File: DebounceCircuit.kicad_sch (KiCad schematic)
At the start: 20 parts, among them U2 74HC14

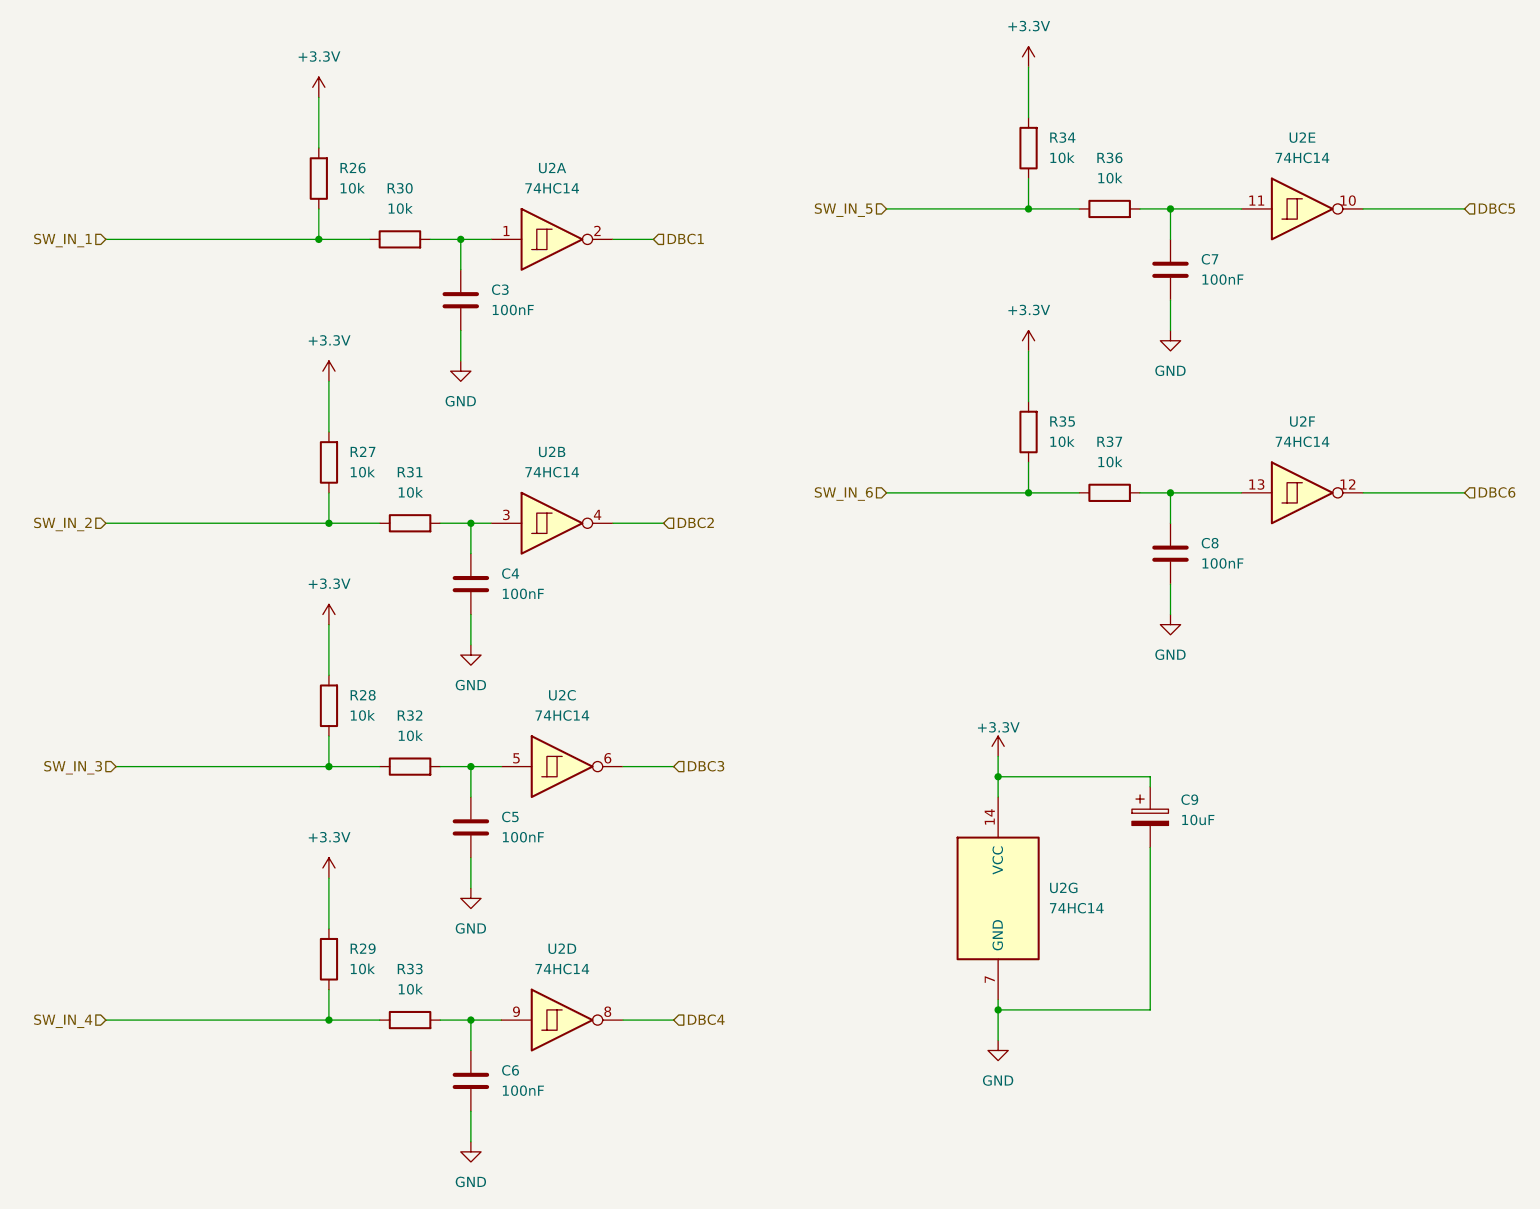
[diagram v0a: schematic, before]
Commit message: Corrigido o botão de seleção de Clock e valores dos capacitores.
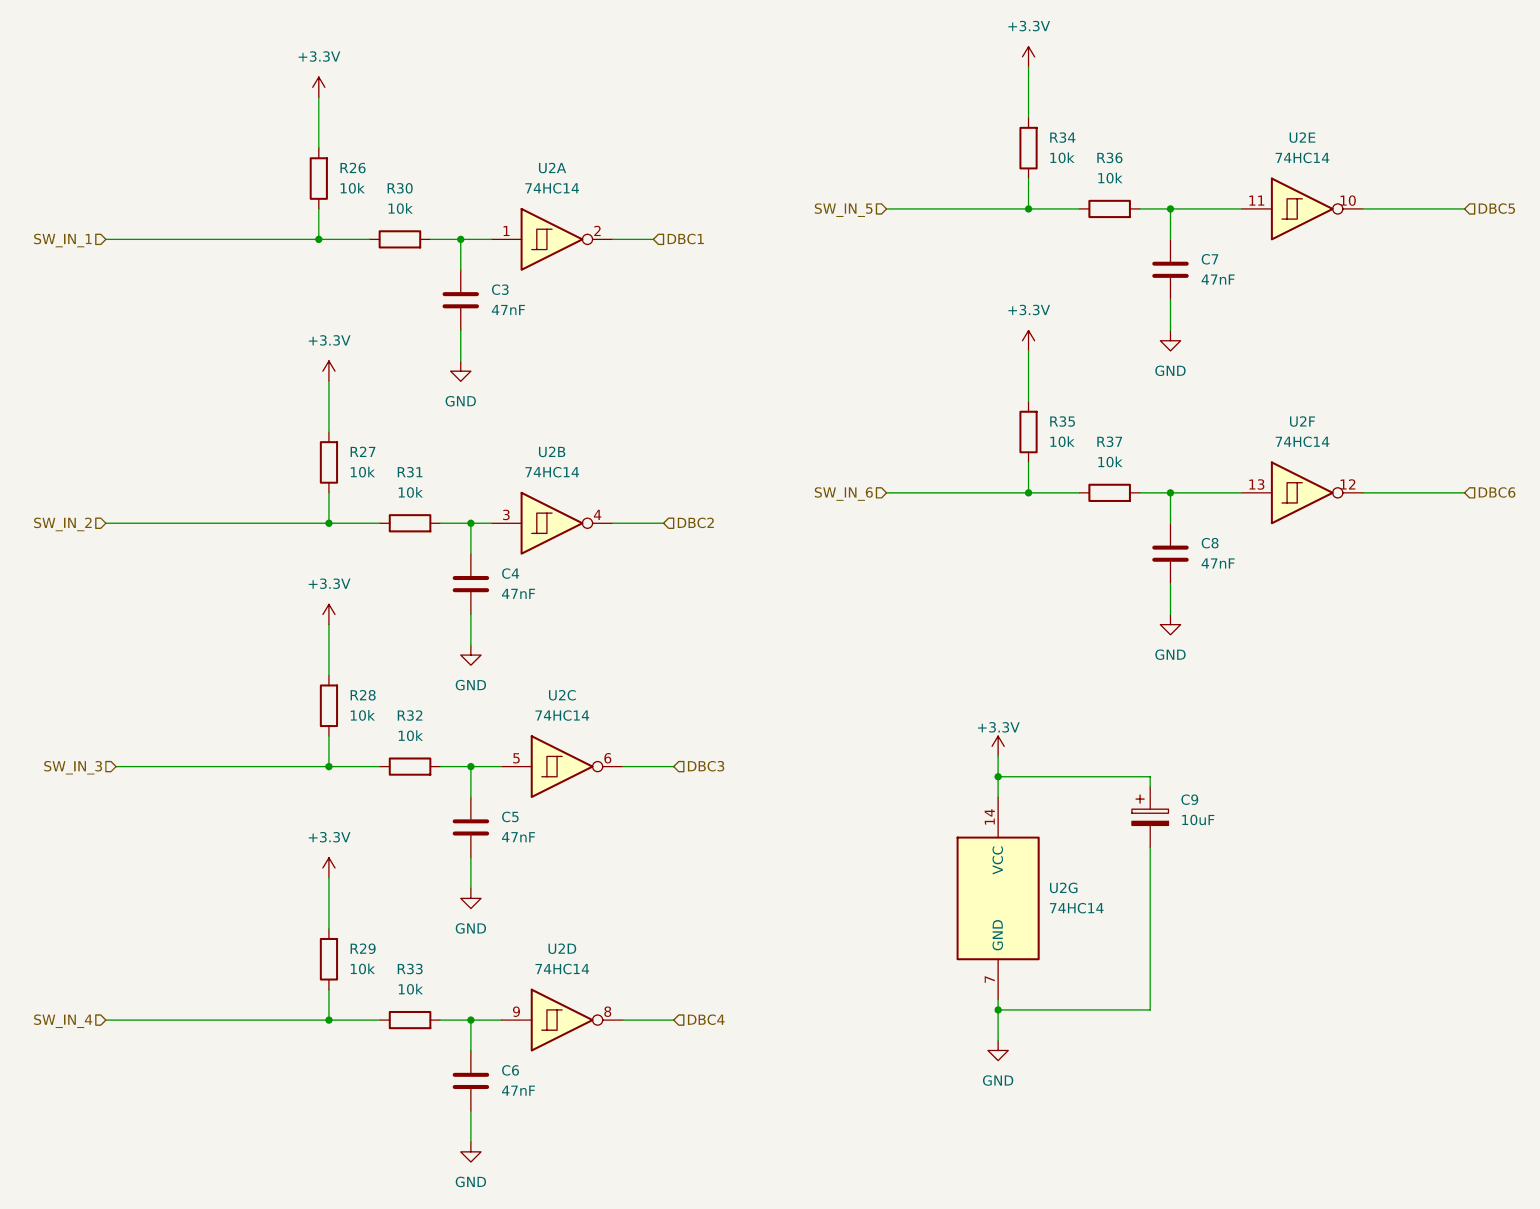
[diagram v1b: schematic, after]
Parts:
- C3, C4, C5, C6, C7, C8: value 100nF -> 47nF
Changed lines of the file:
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@@
       (effects (font (size 1.27 1.27)) (justify left))
     )
-    (property "Value" "100nF" (id 1) (at 190.5 55.8799 0)
+    (property "Value" "47nF" (id 1) (at 190.5 55.8799 0)
       (effects (font (size 1.27 1.27)) (justify left))
     )
@@
       (effects (font (size 1.27 1.27)) (justify left))
     )
-    (property "Value" "100nF" (id 1) (at 190.5 91.4399 0)
+    (property "Value" "47nF" (id 1) (at 190.5 91.4399 0)
       (effects (font (size 1.27 1.27)) (justify left))
     )
@@
       (effects (font (size 1.27 1.27)) (justify left))
     )
-    (property "Value" "100nF" (id 1) (at 102.87 157.4799 0)
+    (property "Value" "47nF" (id 1) (at 102.87 157.4799 0)
       (effects (font (size 1.27 1.27)) (justify left))
     )
@@
       (effects (font (size 1.27 1.27)) (justify left))
     )
-    (property "Value" "100nF" (id 1) (at 101.6 59.6899 0)
+    (property "Value" "47nF" (id 1) (at 101.6 59.6899 0)
       (effects (font (size 1.27 1.27)) (justify left))
     )
@@
       (effects (font (size 1.27 1.27)) (justify left))
     )
-    (property "Value" "100nF" (id 1) (at 102.87 125.7299 0)
+    (property "Value" "47nF" (id 1) (at 102.87 125.7299 0)
       (effects (font (size 1.27 1.27)) (justify left))
     )
@@
       (effects (font (size 1.27 1.27)) (justify left))
     )
-    (property "Value" "100nF" (id 1) (at 102.87 95.2499 0)
-      (effects (font (size 1.27 1.27)) (justify left))
-    )
+    (property "Value" "47nF" (id 1) (at 102.87 95.2499 0)
+      (effects (font (size 1.27 1.27)) (justify left))
+    )

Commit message: Atualizado os valores dos capacitores
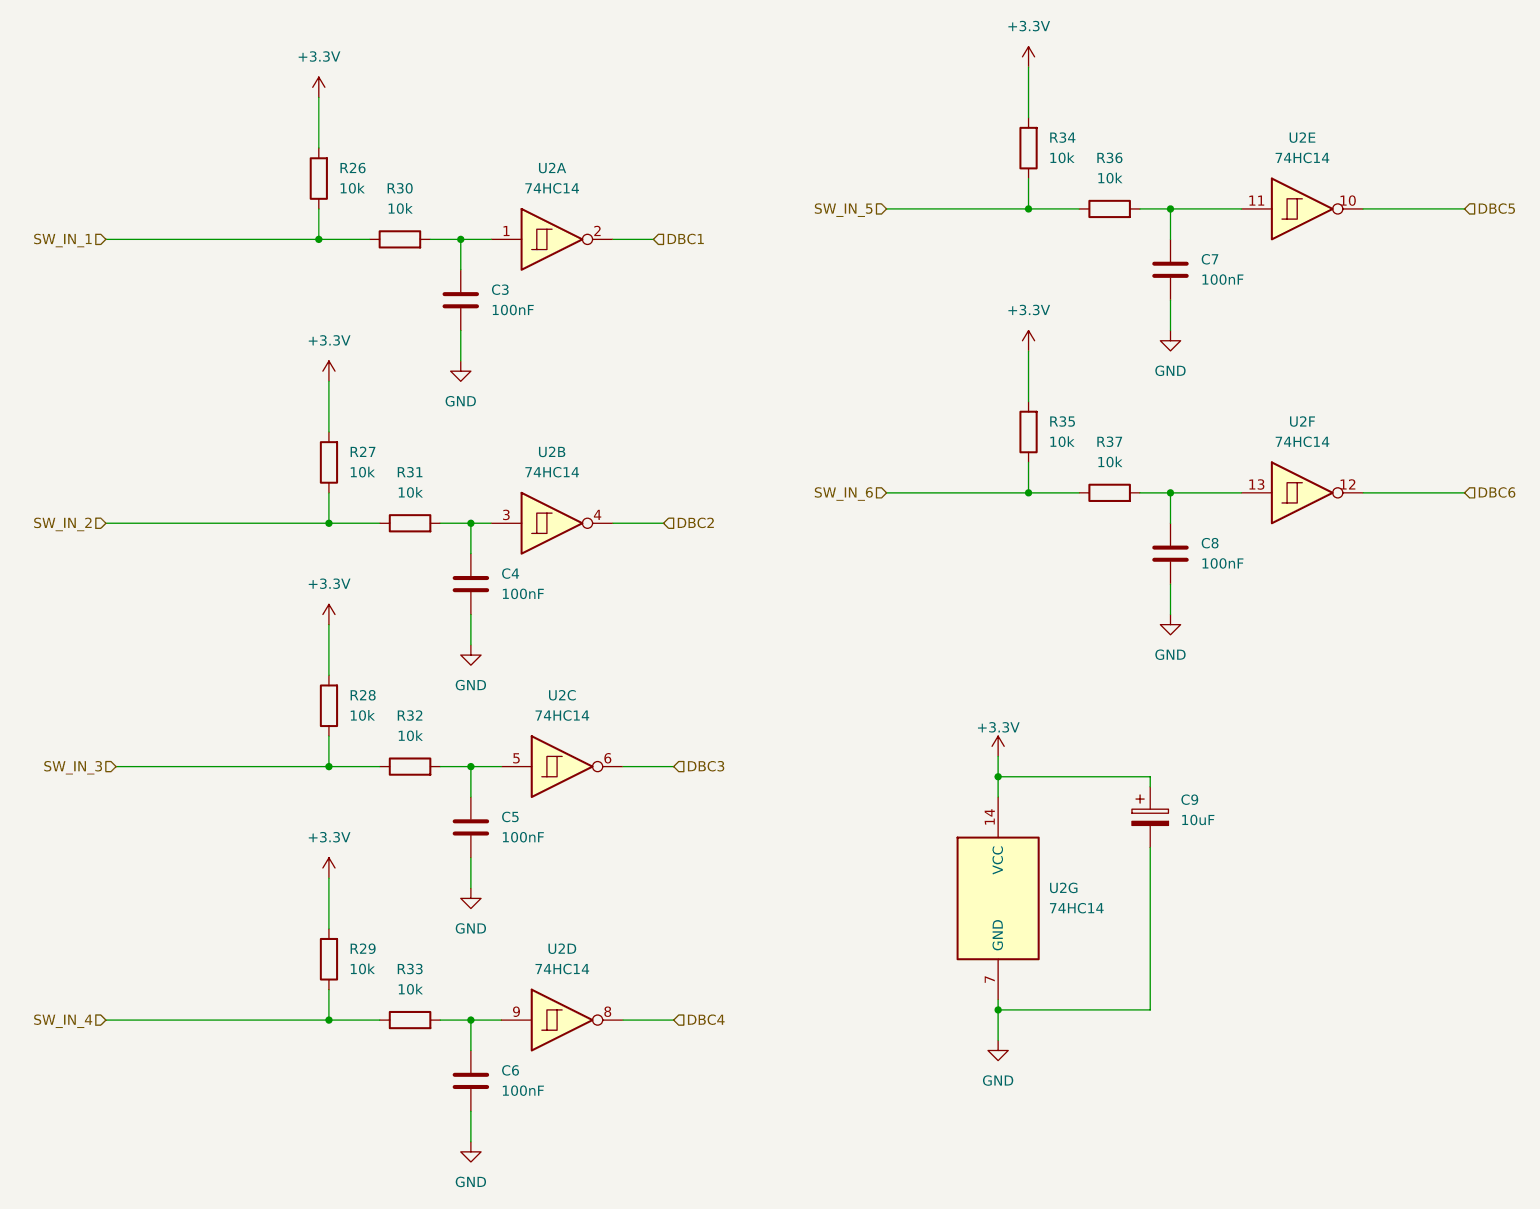
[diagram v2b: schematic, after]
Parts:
- C3, C4, C5, C6, C7, C8: value 47nF -> 100nF
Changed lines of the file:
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@@
       (effects (font (size 1.27 1.27)) (justify left))
     )
-    (property "Value" "47nF" (id 1) (at 190.5 55.8799 0)
+    (property "Value" "100nF" (id 1) (at 190.5 55.8799 0)
       (effects (font (size 1.27 1.27)) (justify left))
     )
@@
       (effects (font (size 1.27 1.27)) (justify left))
     )
-    (property "Value" "47nF" (id 1) (at 190.5 91.4399 0)
+    (property "Value" "100nF" (id 1) (at 190.5 91.4399 0)
       (effects (font (size 1.27 1.27)) (justify left))
     )
@@
       (effects (font (size 1.27 1.27)) (justify left))
     )
-    (property "Value" "47nF" (id 1) (at 102.87 157.4799 0)
+    (property "Value" "100nF" (id 1) (at 102.87 157.4799 0)
       (effects (font (size 1.27 1.27)) (justify left))
     )
@@
       (effects (font (size 1.27 1.27)) (justify left))
     )
-    (property "Value" "47nF" (id 1) (at 101.6 59.6899 0)
+    (property "Value" "100nF" (id 1) (at 101.6 59.6899 0)
       (effects (font (size 1.27 1.27)) (justify left))
     )
@@
       (effects (font (size 1.27 1.27)) (justify left))
     )
-    (property "Value" "47nF" (id 1) (at 102.87 125.7299 0)
+    (property "Value" "100nF" (id 1) (at 102.87 125.7299 0)
       (effects (font (size 1.27 1.27)) (justify left))
     )
@@
       (effects (font (size 1.27 1.27)) (justify left))
     )
-    (property "Value" "47nF" (id 1) (at 102.87 95.2499 0)
-      (effects (font (size 1.27 1.27)) (justify left))
-    )
+    (property "Value" "100nF" (id 1) (at 102.87 95.2499 0)
+      (effects (font (size 1.27 1.27)) (justify left))
+    )
